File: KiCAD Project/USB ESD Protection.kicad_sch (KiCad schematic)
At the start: 5 parts, among them U10 USBLC6-2P6, U11 USBLC6-2P6, U12 USBLC6-2P6, U8 USBLC6-2P6, U9 USBLC6-2P6

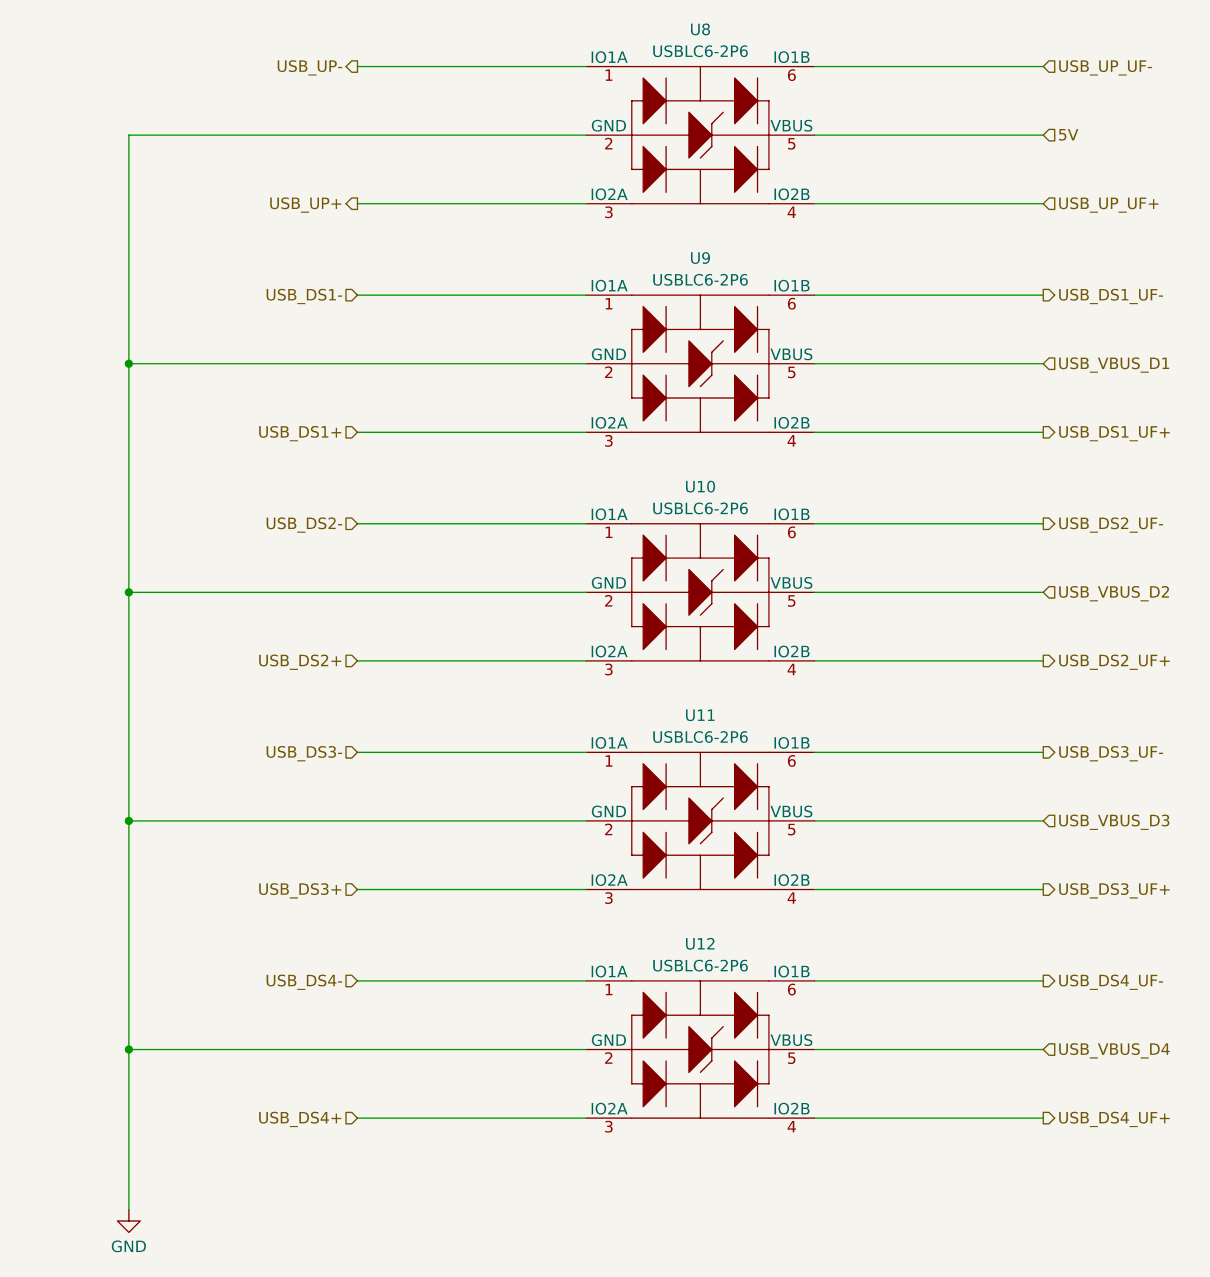
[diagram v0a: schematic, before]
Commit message: v1.0.0 RC2
Build candidate 2
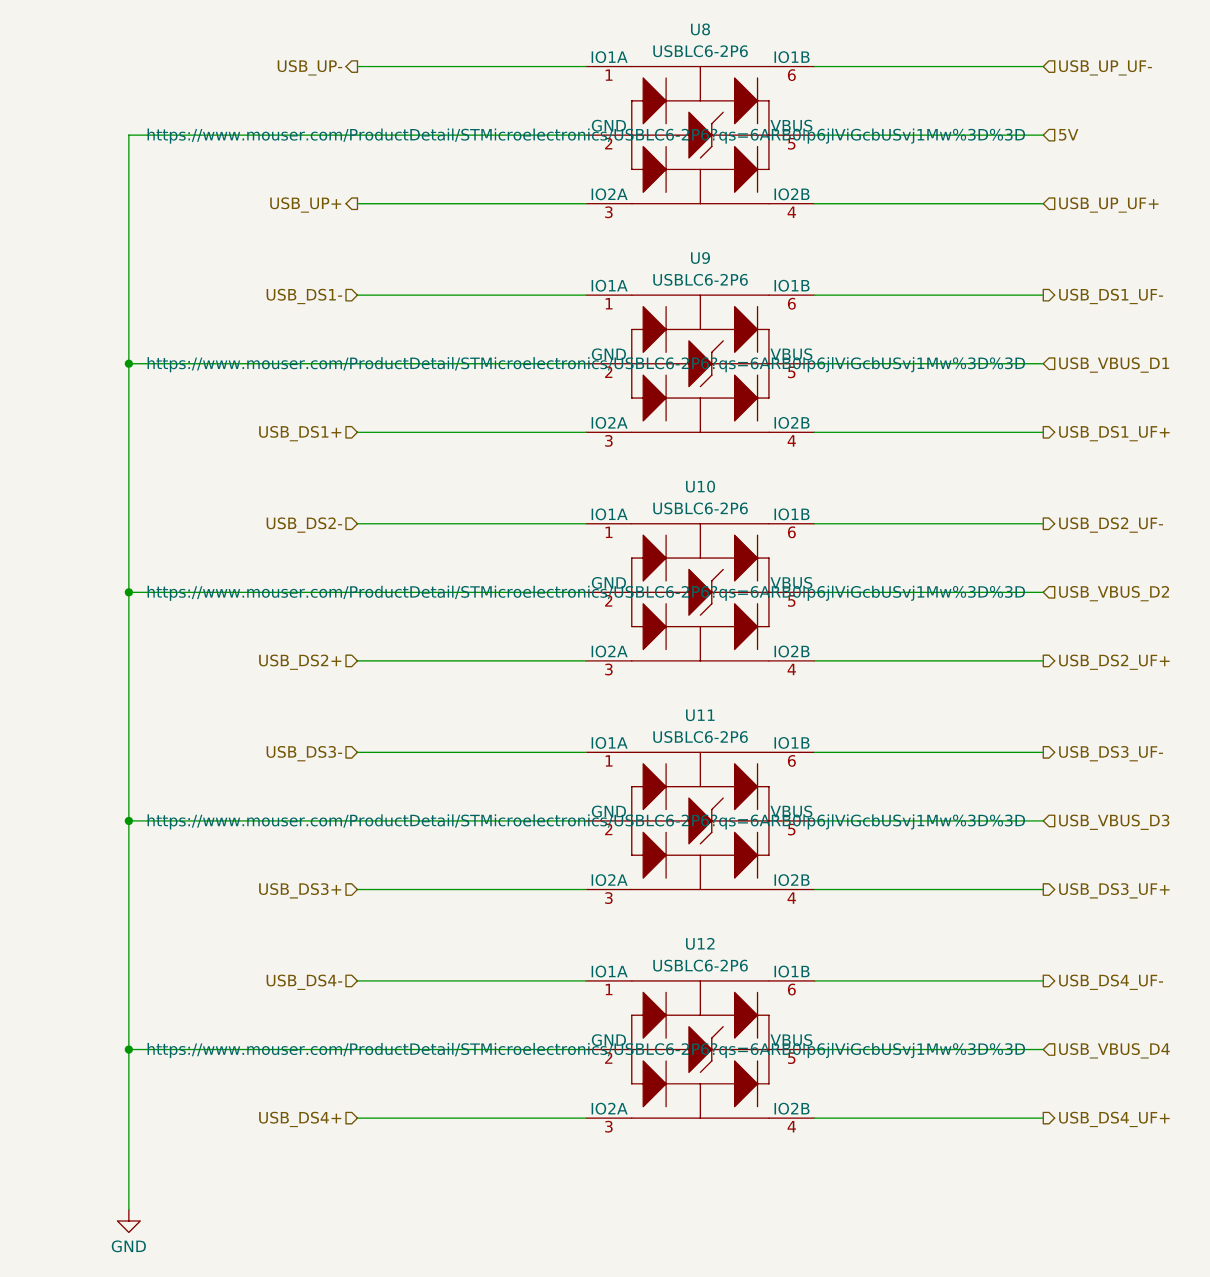
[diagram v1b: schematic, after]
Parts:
- U10, U11, U12, U8, U9: Mouser Price/Stock (none) -> https://www.mouser.com/ProductDetail/STMicroelectronics/USB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
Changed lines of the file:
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@@
+			)
+		)
+		(property "Mouser Price/Stock" "https://www.mouser.com/ProductDetail/STMicroelectronics/USBLC6-2P6?qs=6ARB0lp6jlViGcbUSvj1Mw%3D%3D"
+			(at 127 96.52 0)
+			(effects
+				(font
+					(size 1.27 1.27)
+				)
 			)
 		)
@@
 			)
 		)
+		(property "Mouser Price/Stock" "https://www.mouser.com/ProductDetail/STMicroelectronics/USBLC6-2P6?qs=6ARB0lp6jlViGcbUSvj1Mw%3D%3D"
+			(at 127 147.32 0)
+			(effects
+				(font
+					(size 1.27 1.27)
+				)
+			)
+		)
 		(pin "1"
 		)
@@
 			)
 		)
+		(property "Mouser Price/Stock" "https://www.mouser.com/ProductDetail/STMicroelectronics/USBLC6-2P6?qs=6ARB0lp6jlViGcbUSvj1Mw%3D%3D"
+			(at 127 121.92 0)
+			(effects
+				(font
+					(size 1.27 1.27)
+				)
+			)
+		)
 		(pin "1"
 		)
@@
 			)
 		)
+		(property "Mouser Price/Stock" "https://www.mouser.com/ProductDetail/STMicroelectronics/USBLC6-2P6?qs=6ARB0lp6jlViGcbUSvj1Mw%3D%3D"
+			(at 127 71.12 0)
+			(effects
+				(font
+					(size 1.27 1.27)
+				)
+			)
+		)
 		(pin "1"
 		)
@@
 			)
 		)
+		(property "Mouser Price/Stock" "https://www.mouser.com/ProductDetail/STMicroelectronics/USBLC6-2P6?qs=6ARB0lp6jlViGcbUSvj1Mw%3D%3D"
+			(at 127 45.72 0)
+			(effects
+				(font
+					(size 1.27 1.27)
+				)
+			)
+		)
